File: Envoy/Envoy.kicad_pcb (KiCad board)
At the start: 2 copper layers, 95.5 x 95.4 mm, 53 parts, among them U1 ProMicro

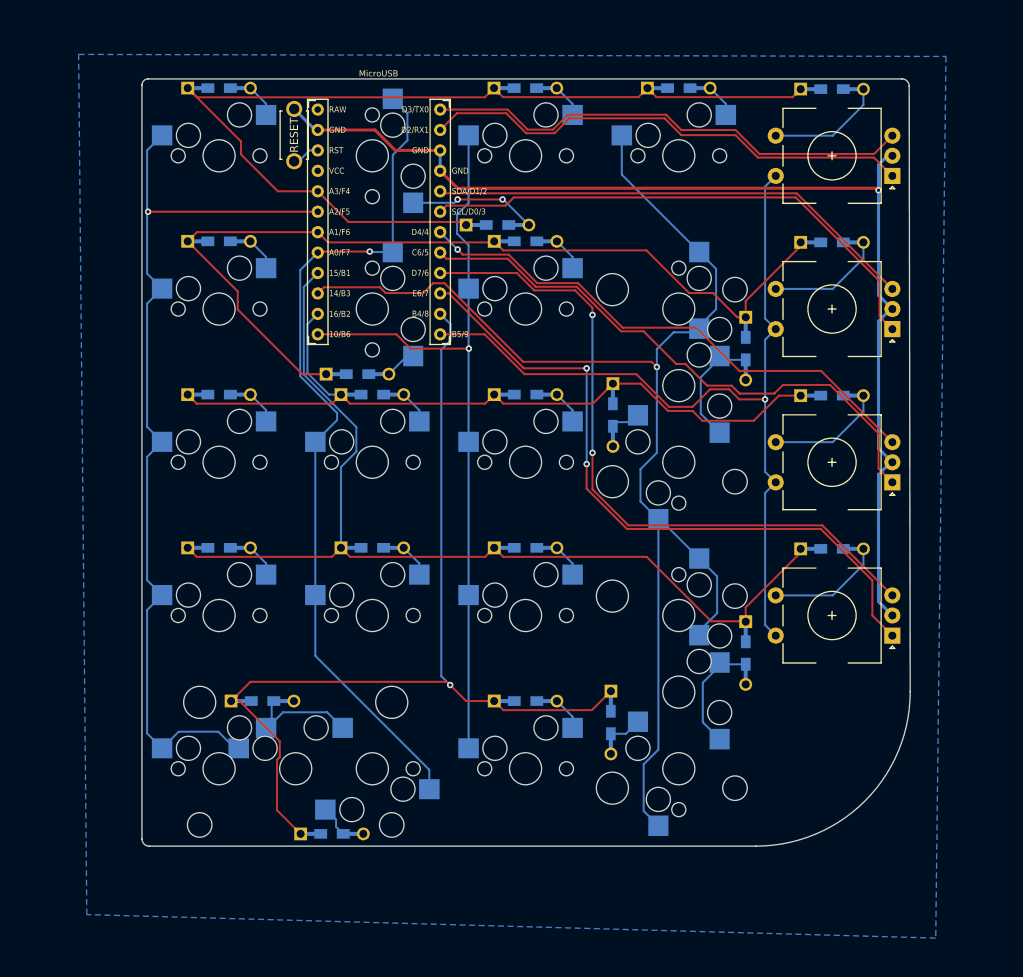
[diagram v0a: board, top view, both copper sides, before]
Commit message: Rev 0.2 including switchplate and backplate
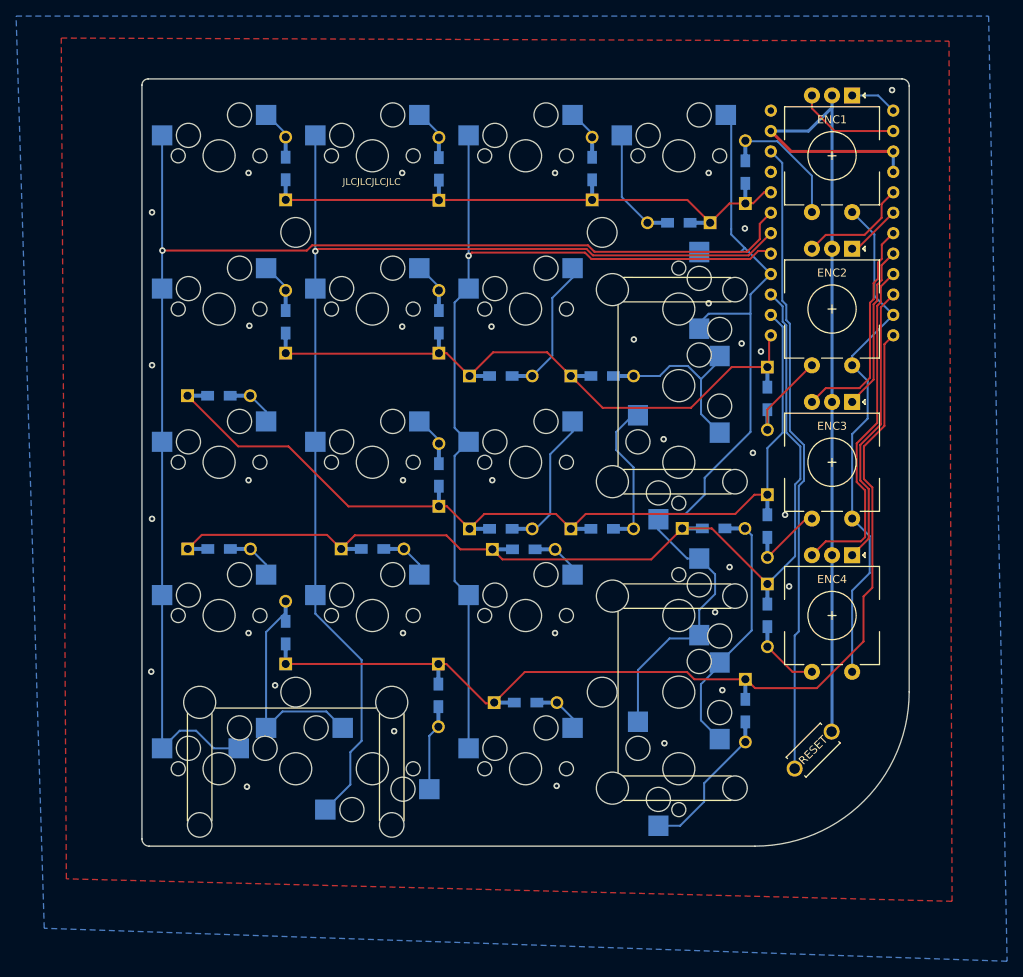
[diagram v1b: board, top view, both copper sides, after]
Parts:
- added H1: MountingHole, Envoy:ClearanceHole_3.7mm, F.Cu at (119.1, 64.3)
- added H2: MountingHole, Envoy:ClearanceHole_3.7mm, F.Cu at (157.2, 64.3)
- added H3: MountingHole, Envoy:ClearanceHole_3.7mm, F.Cu at (119.1, 121.4)
- added H4: MountingHole, Envoy:ClearanceHole_3.7mm, F.Cu at (157.2, 121.4)
- D1, D10, D11, D12, D13, D14, D15, D16, D17, D18, D19, D2, D20, D21, D22, D23, D24, D3, D4, D5, D6, D7, D8, D9: footprint Keebio_parts:Diode-Hybrid-Back -> Envoy:Diode-Hybrid-Back
- ENC1, ENC2: footprint Keebio_parts:RotaryEncoder_EC11 -> Keebio-Parts:RotaryEncoder_EC11-no-legs
- MX1, MX10, MX11, MX13, MX14, MX15, MX19, MX2, MX3, MX5, MX6, MX7, MX9: footprint MX_Only:MXOnly-1U-Hotswap -> Envoy:MXOnly-1U-Hotswap
- MX18, MX20: footprint Envoy:MXOnly-1U-Hotswap-2KeyAlternativeLeft -> Envoy:MXOnly-1U-HotswapReversed-2KeyAlternativeLeft
- MX4: footprint MX_Only:MXOnly-1U-Hotswap -> Envoy:MXOnly-1U-HotswapReversed
- RESET1: footprint kbd:ResetSW -> Envoy:Reset_Jumper_Points
- moved RESET1 100.0 mm to (183.4, 128.7), turned to 45 degrees
- moved ProMicro1 56.3 mm to (185.7, 63.6)
- moved D18 21.7 mm to (136.8, 121.8), turned to 90 degrees
- moved D22 21.0 mm to (177.7, 84.9), turned to 90 degrees
- moved D8 18.2 mm to (157.2, 82.1), turned to 180 degrees
- moved D23 18.1 mm to (177.7, 100.8), turned to 90 degrees
- moved D7 17.0 mm to (144.6, 82.1)
- moved D11 17.0 mm to (144.6, 101.1)
- moved D20 16.8 mm to (175.0, 123.7)
- moved D4 16.7 mm to (166.7, 63.1), turned to 0 degrees
- moved D16 16.0 mm to (171.0, 101.1), turned to 180 degrees
- moved D21 14.9 mm to (175.0, 56.8), turned to -90 degrees
- moved D12 14.2 mm to (157.2, 101.1), turned to 180 degrees
- moved D3 13.0 mm to (155.9, 56.4), turned to -90 degrees
- moved D5 13.0 mm to (117.8, 75.4), turned to -90 degrees
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- renumbered U1 to ProMicro1
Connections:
- ProMicro1 pad 1: enc1B -> enc1A
- ProMicro1 pad 11: row4 -> col4
- ProMicro1 pad 12: col4 -> row4
- ProMicro1 pad 13: col2 -> row1
- ProMicro1 pad 15: col3 -> row3
- ProMicro1 pad 16: row3 -> col3
- ProMicro1 pad 17: col1 -> col2
- ProMicro1 pad 18: row1 -> col1
- ProMicro1 pad 2: enc1A -> enc1B
- RESET1 pad 1: reset -> GND
- RESET1 pad 2: GND -> reset
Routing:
- net reset: track 3.49 -> 78.9 mm
- net enc2A: track 66.3 -> 6.32 mm
- net row0: track 121.6 -> 63.1 mm
- net enc1A: track 61.8 -> 5.89 mm
- net col3: track 165.0 -> 109.4 mm, vias 1 -> 0
- net col0: track 115.0 -> 166.9 mm
- net enc3A: track 71.5 -> 20.5 mm
- net enc4A: track 85.2 -> 35.3 mm, vias 2 -> 0
- net enc1B: track 61.0 -> 12.9 mm
- net enc2B: track 61.2 -> 14.0 mm
- net enc4B: track 86.2 -> 42.6 mm, vias 2 -> 0
- net col4: track 106.0 -> 64.8 mm, vias 1 -> 0
- net row1: track 111.8 -> 71.3 mm
- net col1: track 106.6 -> 146.3 mm
- net enc3B: track 67.0 -> 27.6 mm, vias 1 -> 0
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- added copper zone on F.Cu, net GND
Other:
- board size 95.5 x 95.4 mm -> 95.4 x 95.4 mm
- net class Default removed
- net class Power removed
- rule pad_to_mask_clearance: 0 -> 0.05
- board text added: "1u"
- board text added: "2u"
- board text added: "D0/3"
- board text added: "Envoy by JeJeff rev 0.2"
- board text added: "F5"
- board text added: "F7"
- board text added: "JLCJLCJLCJLC"
